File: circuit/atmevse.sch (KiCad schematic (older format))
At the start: 0 parts

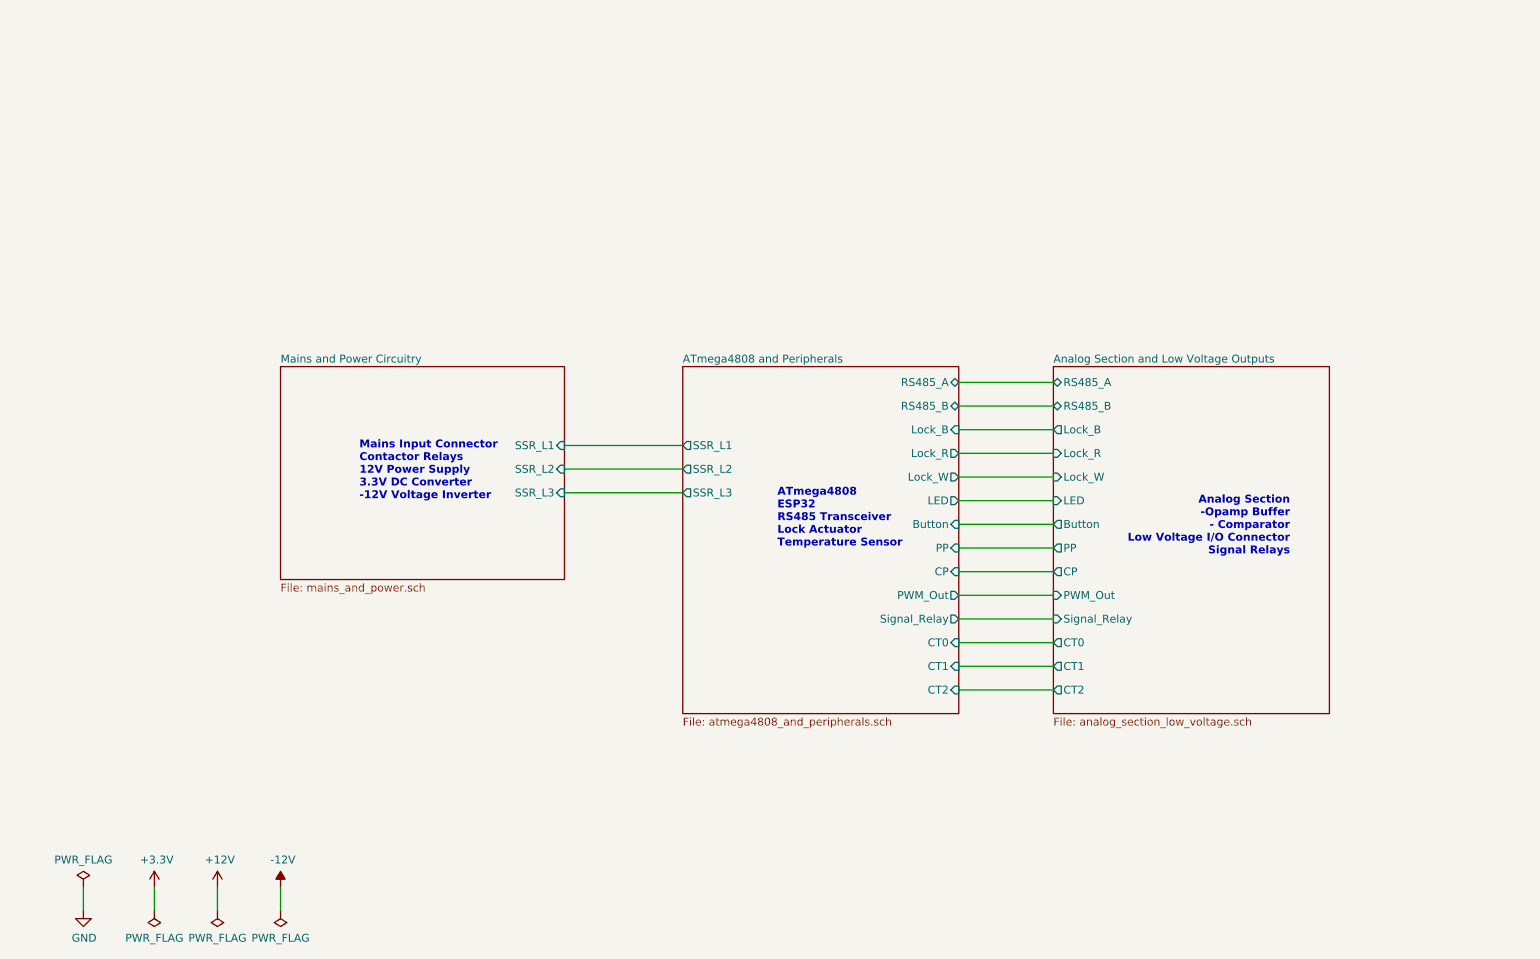
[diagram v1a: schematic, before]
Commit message: Testing build
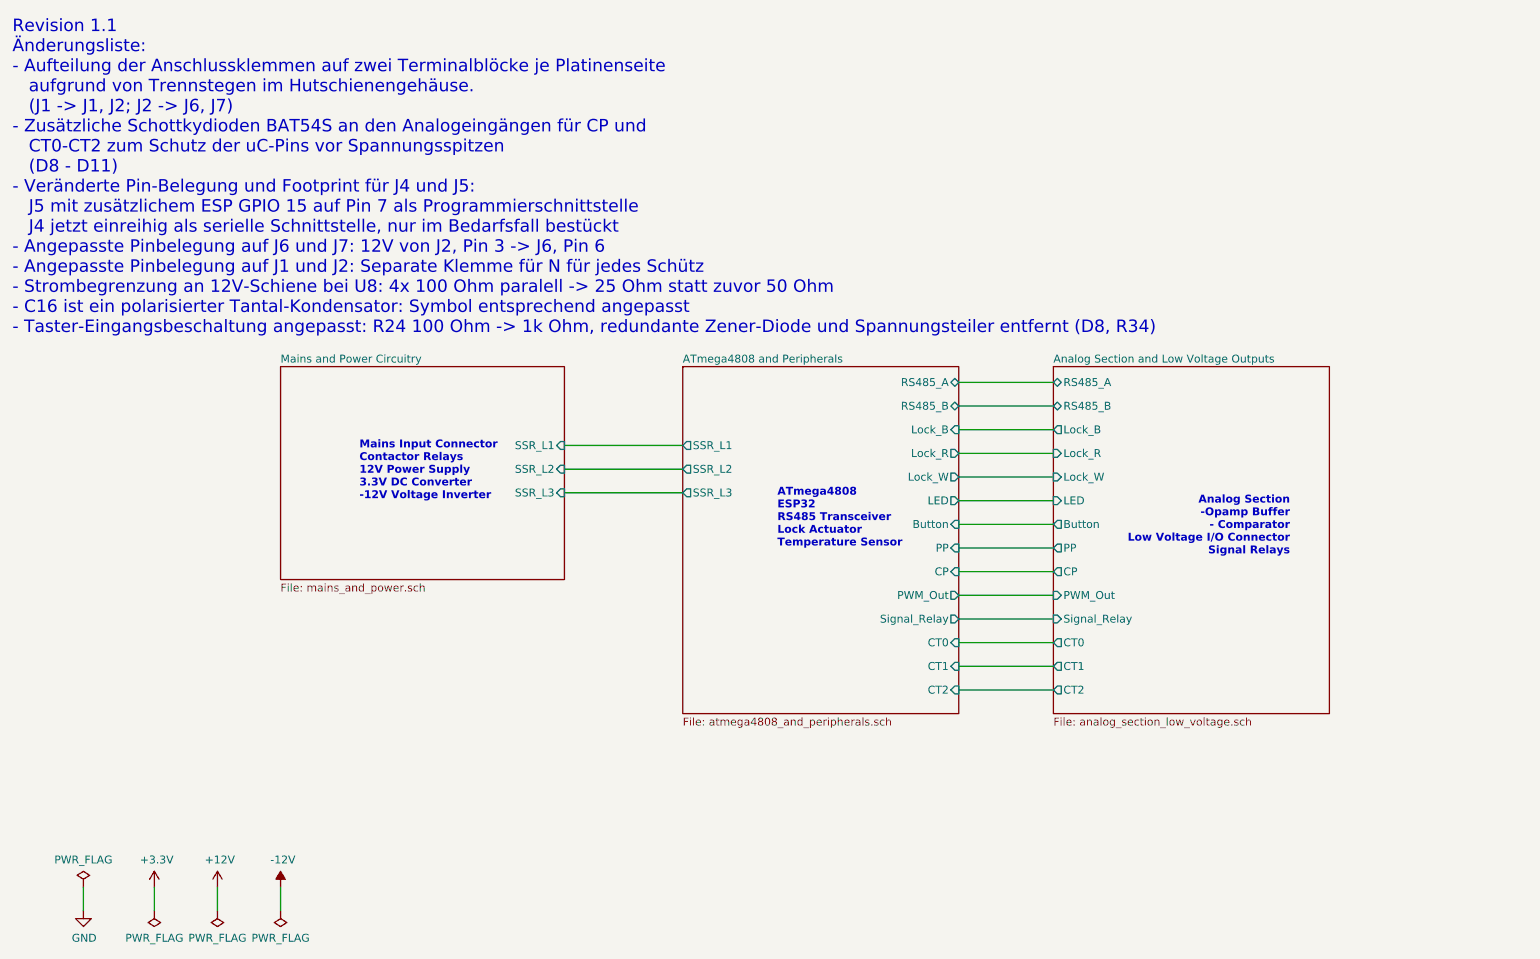
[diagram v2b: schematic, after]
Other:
- note added: "Revision 1.1\nÄnderungsliste:\n- Aufteilung der Anschlussklemmen auf zwei Terminalblöcke je Platinenseite\n aufgrund von Trennstegen im Hutschienengehäuse. \n (J1 -> J1, J2; J2 -> J6, J7)\n- Zusätzliche Schottkydioden BAT54S an den Analogeingängen für CP und \n CT0-CT2 zum Schutz der uC-Pins vor Spannungsspitzen\n (D8 - D11)\n- Veränderte Pin-Belegung und Footprint für J4 und J5: \n J5 mit zusätz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"
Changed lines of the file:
@@
 $Descr A4 11693 8268
 encoding utf-8
-Sheet 1 5
+Sheet 1 4
 Title "FGCCS-Ctrl22"
 Date "2020-08-11"
@@
 Wire Wire Line
 	2300 6000 2300 6150
+Text Notes 600  2500 0    79   ~ 0
+Revision 1.1\nÄnderungsliste:\n- Aufteilung der Anschlussklemmen auf zwei Terminalblöcke je Platinenseite\n   aufgrund von Trennstegen im Hutschienengehäuse. \n   (J1 -> J1, J2; J2 -> J6, J7)\n- Zusätzliche Schottkydioden BAT54S an den Analogeingängen für CP und \n   CT0-CT2 zum Schutz der uC-Pins vor Spannungsspitzen\n   (D8 - D11)\n- Veränderte Pin-Belegung und Footprint für J4 und J5: \n   J5 mit zusätzlichem ESP GPIO 15 auf Pin 7 als Programmierschnittstelle\n   J4 jetzt einreihig als serielle Schnittstelle, nur im Bedarfsfall bestückt\n- Angepasste Pinbelegung auf J6 und J7: 12V von J2, Pin 3 -> J6, Pin 6\n- Angepasste Pinbelegung auf J1 und J2: Separate Klemme für N für jedes Schütz\n- Strombegrenzung an 12V-Schiene bei U8: 4x 100 Ohm paralell -> 25 Ohm statt zuvor 50 Ohm \n- C16 ist ein polarisierter Tantal-Kondensator: Symbol entsprechend angepasst\n- Taster-Eingangsbeschaltung angepasst: R24 100 Ohm -> 1k Ohm, redundante Zener-Diode und Spannungsteiler entfernt (D8, R34)
 $EndSCHEMATC
